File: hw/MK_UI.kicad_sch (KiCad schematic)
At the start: 34 parts, among them J11 Conn_01x03, J3 Conn_02x10_Odd_Even, J4 Conn_01x07, J7 Conn_01x20, SW2 UP, SW3 RT, SW4 DN, SW5 LF, SW6 EN

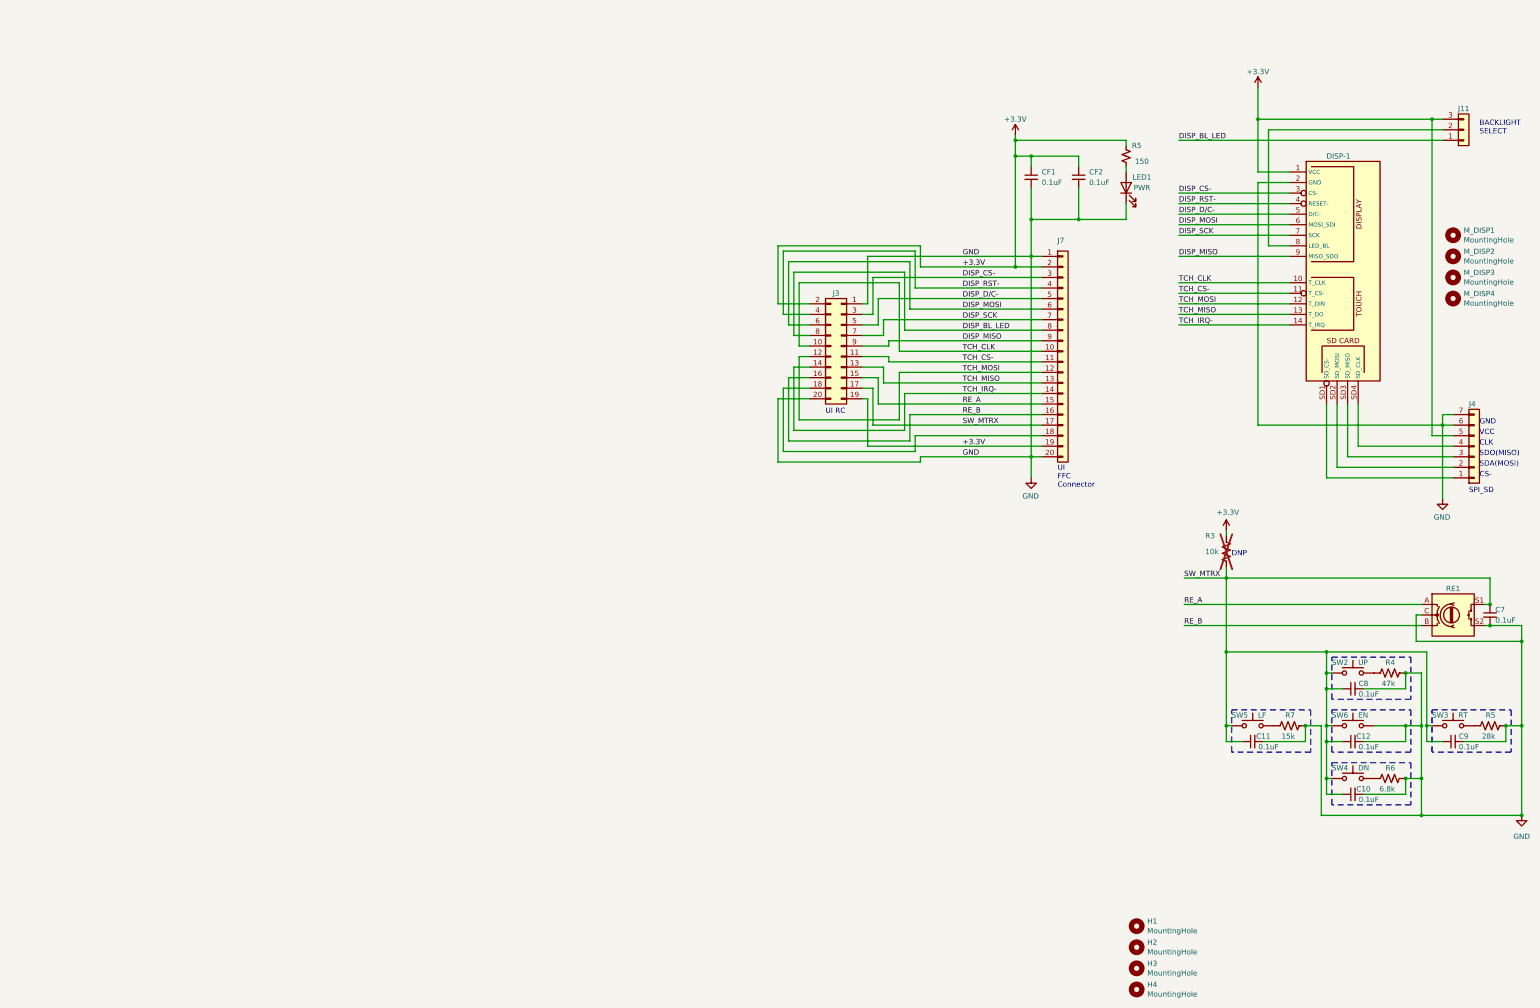
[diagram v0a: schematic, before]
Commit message: Electrical checks complete.
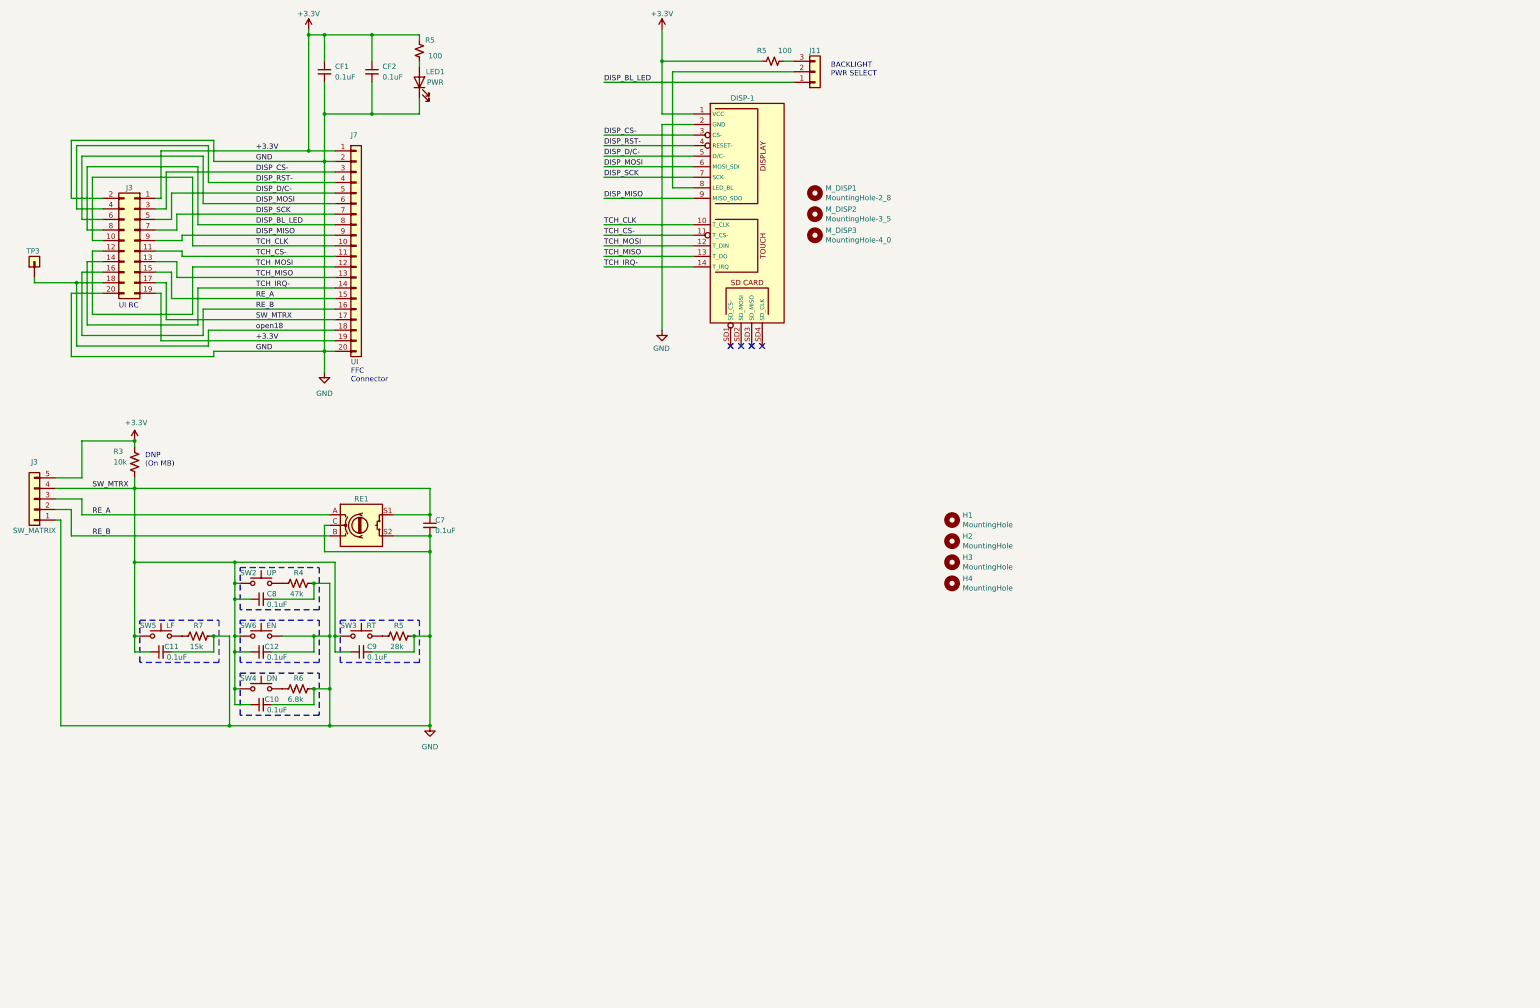
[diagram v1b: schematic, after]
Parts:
- removed J4: Conn_01x07, symbol Connector_Generic:Conn_01x07
- removed M_DISP4: MountingHole, MountingHole:MountingHole_2.7mm_M2.5, symbol Mechanical:MountingHole
- added J3: SW_MATRIX, symbol Connector_Generic:Conn_01x05
- added R5: 100, Resistor_THT:R_Axial_DIN0207_L6.3mm_D2.5mm_P10.16mm_Horizontal, symbol Device:R_Small_US
- added TP3: Test_Point_01, symbol Test_point_Jump:TP_01
- M_DISP1: value MountingHole -> MountingHole-2_8
- M_DISP2: value MountingHole -> MountingHole-3_5
- M_DISP3: value MountingHole -> MountingHole-4_0
- R3: now fitted
- R5: value 150 -> 100
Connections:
- net +3.3V: now also J3.1 (Pin_1), J7.1 (Pin_1), J3.5 (Pin_5), R5.1; no longer J11.3 (Pin_3), J3.2 (Pin_2), J7.2 (Pin_2)
- net GND: now also J3.2 (Pin_2), J7.2 (Pin_2), J3.1 (Pin_1); no longer J3.1 (Pin_1), J7.1 (Pin_1)
- net RE_A: now also J3.3 (Pin_3)
- net RE_B: now also J3.2 (Pin_2)
- net SW_MTRX: now also J3.4 (Pin_4)
- net open18: now reaches J3.18 (Pin_18), J7.18 (Pin_18)
- net open18: now also TP3.1 (Pin_1)
- new net: J11.3 (Pin_3), R5.2
- no-connect marks 0 -> 4
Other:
- note added: "BACKLIGHT PWR SELECT"
- note added: "DNP (On MB)"
- note removed: "BACKLIGHT SELECT"
- note removed: "CLK"
- note removed: "CS-"
- note removed: "DNP"
- note removed: "GND"
- note removed: "SDA(MOSI)"
- note removed: "SDO(MISO)"
- note removed: "SPI_SD"
- note removed: "VCC"
- moved on the sheet: C10, C11, C12, C7, C8, C9, CF1, CF2, DISP-1, H1, H2, H3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
